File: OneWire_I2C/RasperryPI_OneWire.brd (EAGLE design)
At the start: 63.5 x 50.8 mm, 47 parts, among them P1 MOLEX_MINILITE_TRAP_2, P2 MOLEX_MINILITE_TRAP_2, P3 MOLEX_MINILITE_TRAP_2, T1 BC817, T2 BC817, U1 P82B715D, U2 DS2482-800

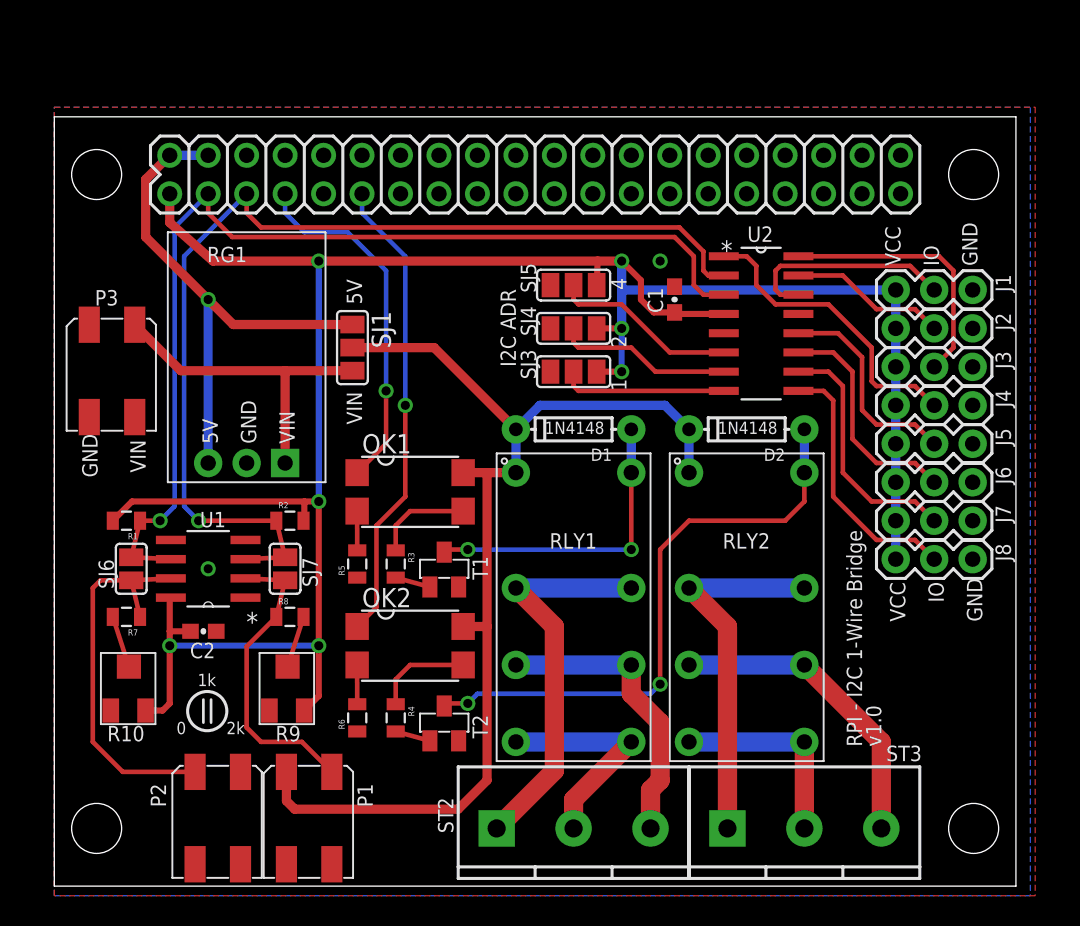
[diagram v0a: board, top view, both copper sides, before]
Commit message: Gate 4, and misc updates
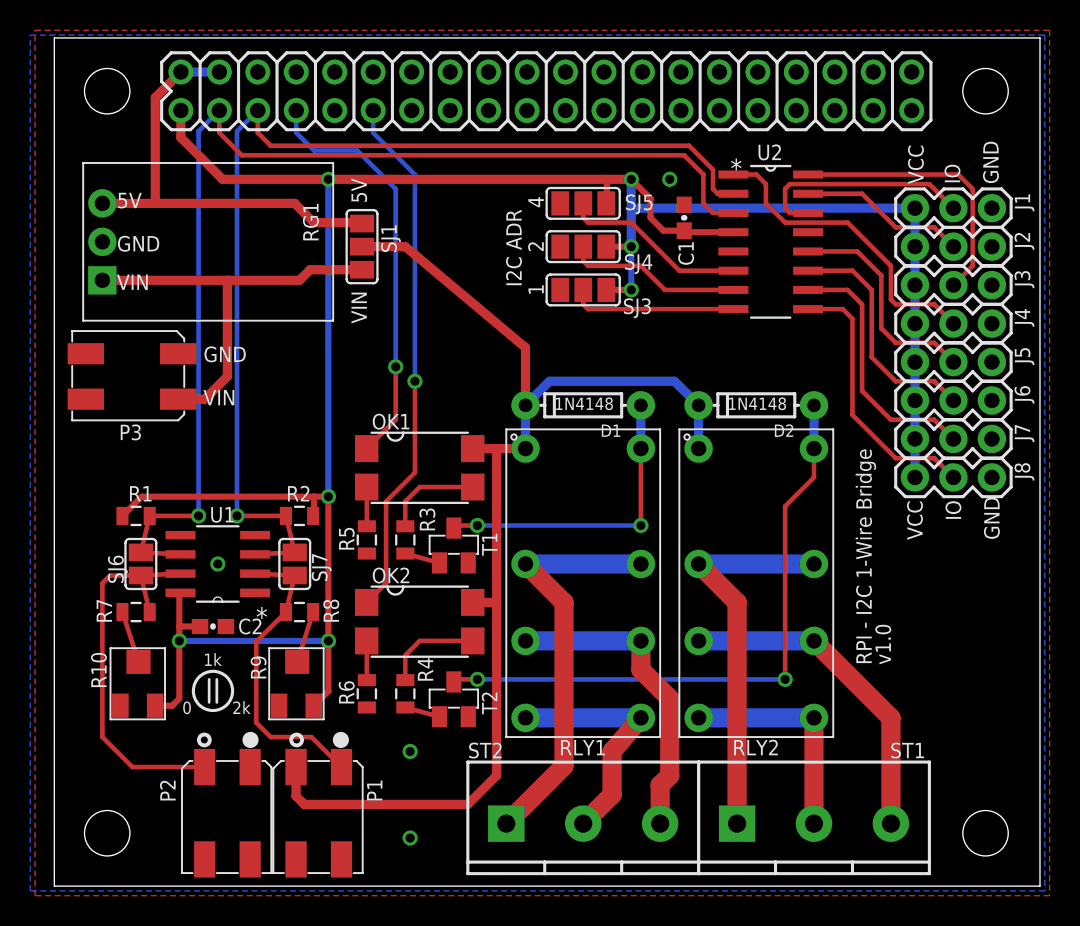
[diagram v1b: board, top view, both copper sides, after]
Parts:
- removed ST3: (no value), Puffin:SCREWTERM_0.2X3
- removed U$1, U$2, U$3, U$4: (no value), SparkFun-Electromechanical:STAND-OFF
- added ST1: (no value), Puffin:SCREWTERM_0.2X3
- added U$6: (no value), Puffin:RPI_BOARD
- moved RG1 17.4 mm to (3.17, 42.5), turned to 270 degrees
- moved SJ1 6.70 mm to (20.3, 42.2)
- moved PI 5.55 mm to (32.5, 52.5)
- moved J1 5.54 mm to (56.8, 44.8)
- moved J2 5.54 mm to (56.8, 42.2)
- moved J3 5.54 mm to (56.8, 39.7)
- moved J4 5.54 mm to (56.8, 37.1)
- moved J5 5.54 mm to (56.8, 34.6)
- moved J6 5.54 mm to (56.8, 32.1)
- moved J7 5.54 mm to (56.8, 29.5)
- moved J8 5.54 mm to (56.8, 27.0)
- moved C1 5.43 mm to (41.6, 44.1)
- moved SJ3 5.43 mm to (34.9, 39.4)
- moved SJ4 5.43 mm to (34.9, 42.2)
- moved SJ5 5.43 mm to (34.9, 45.1)
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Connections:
- net N$17: now also ST1.1; no longer ST3.1
- net N$18: now also ST1.3; no longer ST3.3
- net N$19: now also ST1.2; no longer ST3.2
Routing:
- net SDA: track 68.0 -> 74.4 mm
- net 12V: track 21.7 -> 27.7 mm
- net 5V: track 35.4 -> 29.6 mm, vias 1 -> 0
- net 3.3V: track 155.2 -> 160.9 mm
- net VCC: track 73.4 -> 78.6 mm
- net RLY1: track 23.6 -> 27.5 mm
- net RLY2: track 31.1 -> 34.9 mm
- net SCL: track 69.2 -> 71.0 mm
- net N$13: track 39.3 -> 40.8 mm
- net N$20: track 26.1 -> 27.4 mm
- net N$21: track 19.5 -> 20.7 mm
- net N$19: track 13.3 -> 14.6 mm
- net N$18: track 20.5 -> 21.8 mm
- net N$17: track 24.5 -> 25.8 mm
- net N$22: track 14.9 -> 16.1 mm
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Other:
- board size 63.5 x 50.8 mm -> 65.1 x 56 mm
